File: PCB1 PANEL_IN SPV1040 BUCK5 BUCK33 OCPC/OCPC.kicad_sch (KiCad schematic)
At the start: 35 parts, among them J11 Conn_01x02_Pin, J12 Conn_01x02_Pin, J13 OCPC_EN, J14 OCPC_EN, J15 OCPC_EN, J16 OCPC_EN, J17 OCPC_EN, J7 Conn_01x02_Pin, J8 Conn_01x02_Pin, J9 Conn_01x02_Pin, U14 TPS2557DRBR, U16 TPS2557DRBR, U17 TPS2557DRBR, U18 TPS2557DRBR, U19 TPS2557DRBR

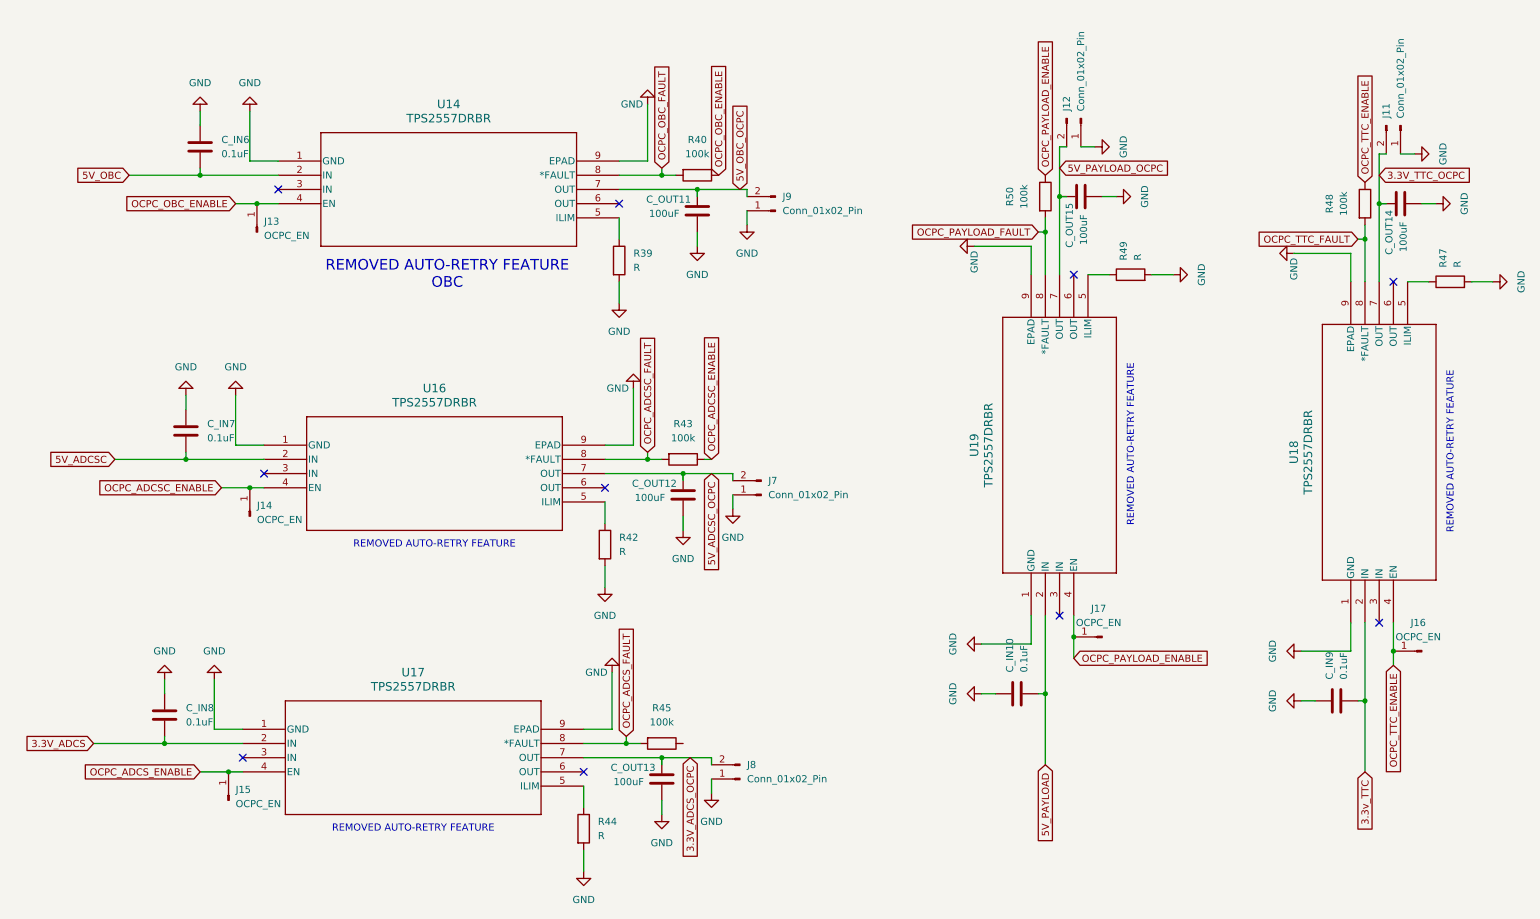
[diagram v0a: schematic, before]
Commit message: VCOMMIT
EDITS N+I
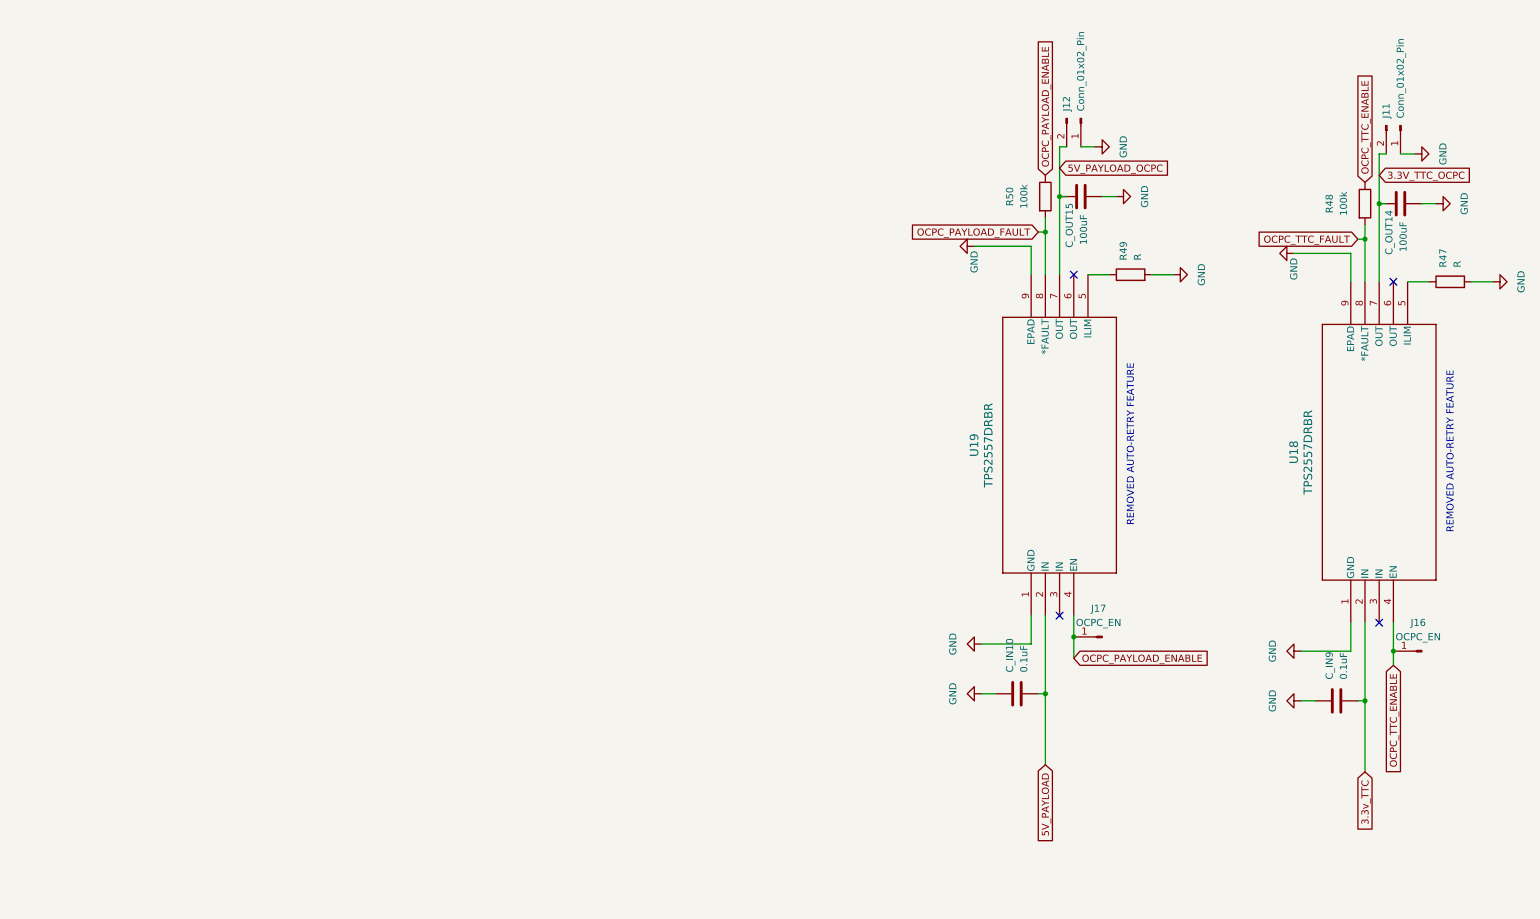
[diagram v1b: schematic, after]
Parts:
- removed C_IN6, C_IN7, C_IN8: 0.1uF, Capacitor_SMD:C_0603_1608Metric, symbol Device:C
- removed C_OUT11, C_OUT12, C_OUT13: 100uF, Capacitor_SMD:C_0504_1310Metric, symbol Device:C
- removed J13, J14, J15: OCPC_EN, symbol Connector:Conn_01x01_Pin
- removed J7, J8, J9: Conn_01x02_Pin, Connector_PinHeader_2.54mm:PinHeader_1x02_P2.54mm_Vertical, symbol Connector:Conn_01x02_Pin
- removed R39, R42, R44: R, Resistor_SMD:R_0603_1608Metric_Pad0.98x0.95mm_HandSolder, symbol Device:R
- removed R40, R43, R45: 100k, Resistor_SMD:R_01005_0402Metric_Pad0.57x0.30mm_HandSolder, symbol Device:R
- removed U14, U16, U17: TPS2557DRBR, TPS2557:DRB8_2P4X1P65, symbol TPS2557:TPS2557DRBR
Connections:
- no-connect marks 10 -> 4
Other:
- note removed: "REMOVED AUTO-RETRY FEATURE OBC"
